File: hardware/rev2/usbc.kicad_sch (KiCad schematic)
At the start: 39 parts, among them J1 UART, J3 USB_C_Receptacle_USB2.0, J8 Conn_01x04_Socket, J9 Conn_01x03_Socket, SW4 PB400EEQR1BLK, SW5 FTDI/DIRECT, SW6 SWx02, U11 FT2232HL, U7 AP63203WU, U8 AP2114H-2.5TRG1, Y1 12MHz

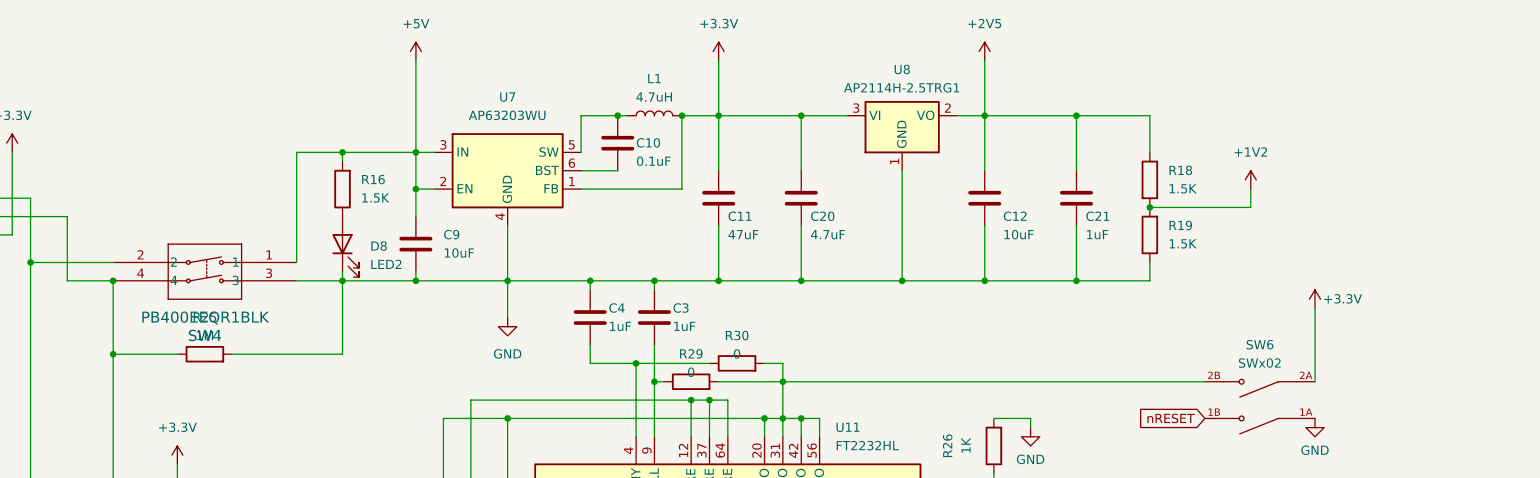
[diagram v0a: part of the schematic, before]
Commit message: rev2, clocks
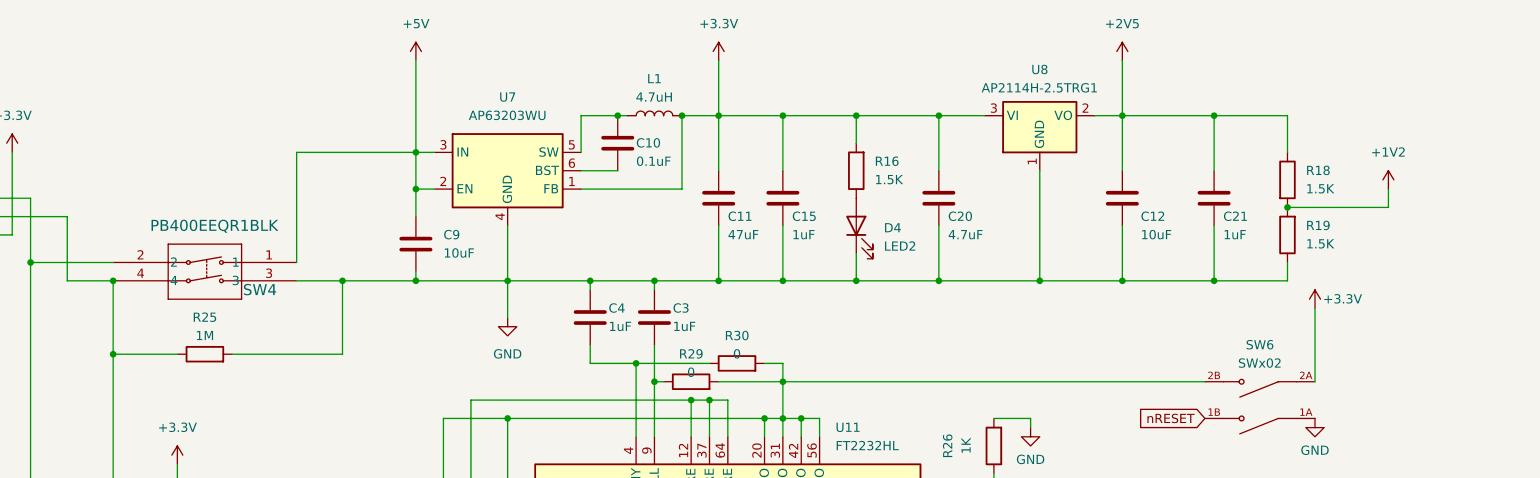
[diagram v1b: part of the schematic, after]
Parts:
- added C15: 1uF, Capacitor_SMD:C_0603_1608Metric, symbol Device:C
- D4: renamed from D8; footprint LED_THT:LED_D3.0mm -> LED_SMD:LED_0603_1608Metric
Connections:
- net +3.3V: now also R16.2, C15.1
- net +5V: no longer R16.2
- net GND: now also C15.2
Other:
- moved on the sheet: C12, C20, C21, D4, R16, R18, R19, U8
